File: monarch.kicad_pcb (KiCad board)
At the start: 2 copper layers, 159.6 x 123.3 mm, 137 parts, among them J1 USB_C_Receptacle_USB2.0, J2 USB_C_Receptacle_USB2.0, J3 OLED, SW1 SW_PUSH, SW10 SW_PUSH, SW11 SW_PUSH, SW12 SW_PUSH, SW13 SW_PUSH, SW14 SW_PUSH, SW15 SW_PUSH, SW16 SW_PUSH, SW17 SW_PUSH, SW18 SW_PUSH, SW19 Rotary_Encoder, SW2 SW_PUSH, SW20 SW_PUSH, SW21 SW_PUSH, SW22 SW_PUSH, SW23 SW_PUSH, SW24 SW_PUSH, SW3 SW_PUSH, SW4 SW_PUSH, SW5 SW_PUSH, SW6 SW_PUSH, SW7 SW_PUSH, SW8 SW_PUSH, SW9 SW_PUSH, U1 ATMEGA32U4, U2 MIC5219-5.0YMM, X1 16Mhz

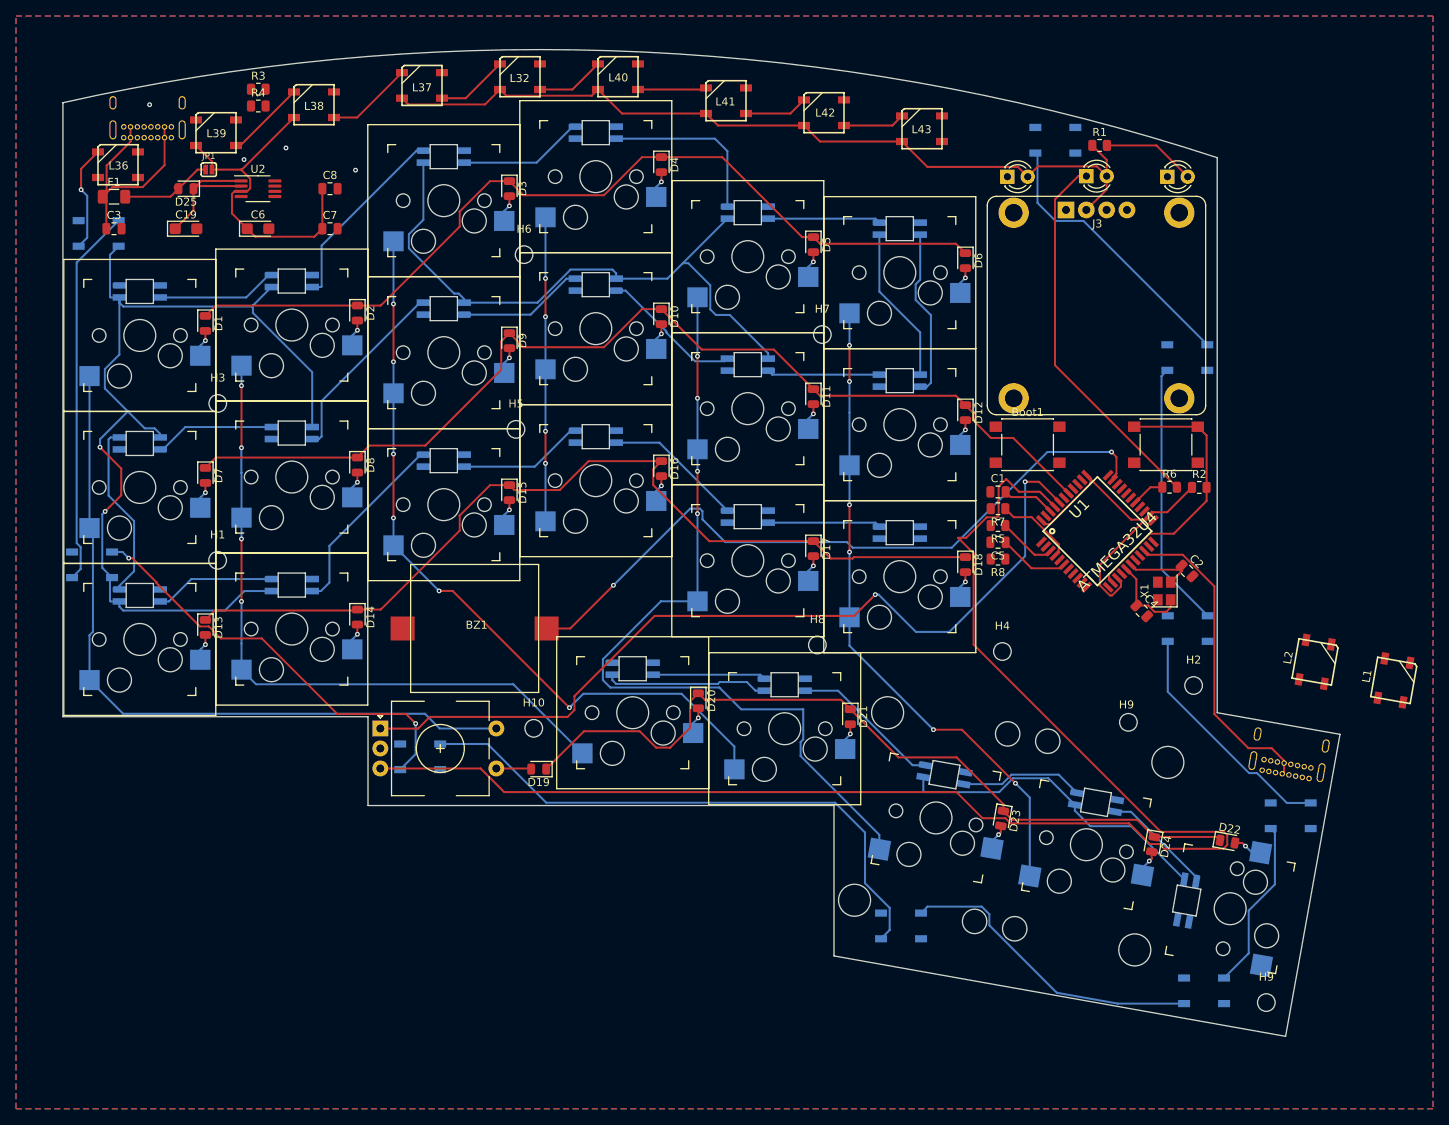
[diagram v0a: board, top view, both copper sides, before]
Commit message: plate edge case
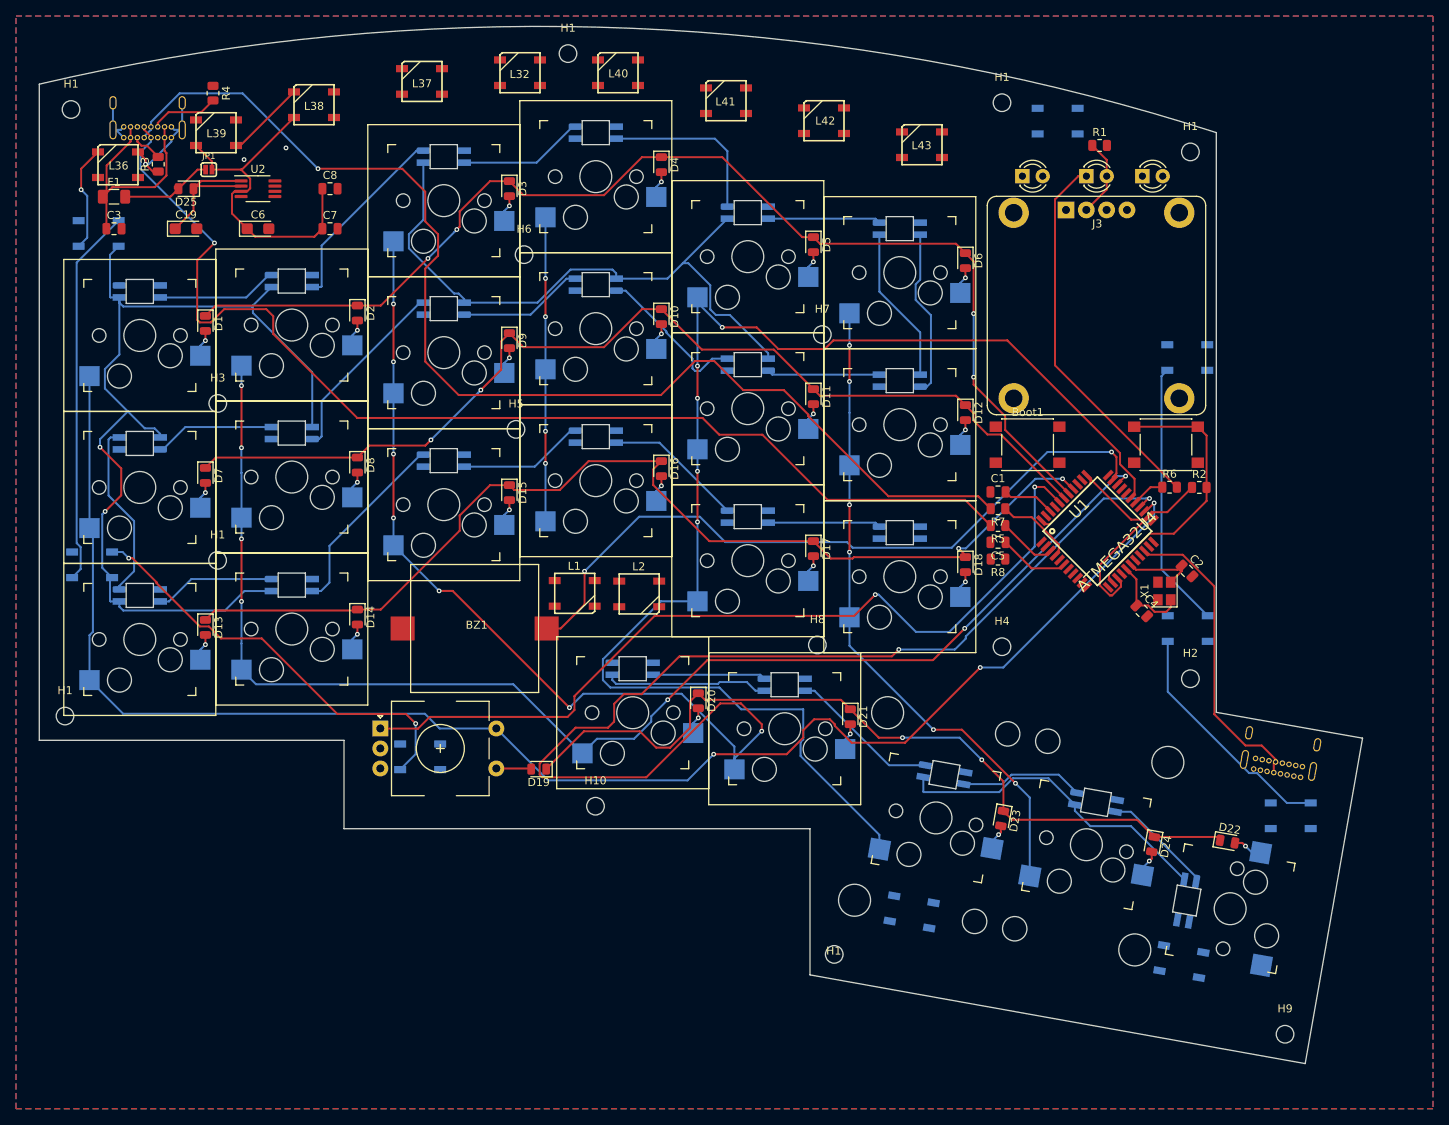
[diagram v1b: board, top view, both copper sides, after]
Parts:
- removed the H9 at (165.0, 126.7)
- removed the H9 at (147.8, 91.7)
- added H1: Hole, MountingHole:MountingHole_2.2mm_M2, F.Cu at (132.0, 14.2)
- added H1: Hole, MountingHole:MountingHole_2.2mm_M2, F.Cu at (155.6, 20.4)
- added H1: Hole, MountingHole:MountingHole_2.2mm_M2, F.Cu at (111.0, 120.7)
- added H1: Hole, MountingHole:MountingHole_2.2mm_M2, F.Cu at (14.9, 90.9)
- added H1: Hole, MountingHole:MountingHole_2.2mm_M2, F.Cu at (15.6, 15.1)
- added H1: Hole, MountingHole:MountingHole_2.2mm_M2, F.Cu at (77.8, 8.11)
- added H9: Hole, MountingHole:MountingHole_2.2mm_M2, F.Cu at (167.4, 130.7)
- moved L1 103.0 mm to (78.6, 75.6), turned to 0 degrees
- moved L2 84.9 mm to (86.7, 75.7), turned to 0 degrees
- moved R3 15.6 mm to (26.5, 21.9), turned to 90 degrees
- moved H10 12.4 mm to (81.2, 102.2)
- moved R4 5.89 mm to (33.4, 13.1), turned to 270 degrees
- moved L7 4.63 mm to (154.4, 121.6), turned to 350 degrees
- moved RED1 3.13 mm to (149.6, 23.4)
- moved L3 2.41 mm to (138.9, 16.6)
- moved L8 2.20 mm to (120.7, 115.4), turned to 350 degrees
- moved L43 2.00 mm to (122.0, 19.5)
- moved D26 1.88 mm to (134.6, 23.4)
- moved J2 1.07 mm to (163.5, 97.5)
- moved L42 1.00 mm to (109.8, 16.5)
- moved H2 0.94 mm to (155.6, 86.2)
- moved H4 0.60 mm to (132.0, 82.2)
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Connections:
- D1 pad 1: A3 -> A2
- D10 pad 1: A2 -> A3
- D11 pad 1: A2 -> A3
- D12 pad 1: A2 -> A3
- D2 pad 1: A3 -> A2
- D3 pad 1: A3 -> A2
- D4 pad 1: A3 -> A2
- D5 pad 1: A3 -> A2
- D6 pad 1: A3 -> A2
- D7 pad 1: A2 -> A3
- D8 pad 1: A2 -> A3
- D9 pad 1: A2 -> A3
- J2 pad A5: +5V -> GND
- J2 pad B5: +5V -> GND
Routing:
- net A5: track 185.9 -> 0.00 mm
- net Net-(J1-PadA6): track 0.00 -> 147.7 mm, vias 0 -> 1
- net Net-(J1-PadA7): track 0.00 -> 142.3 mm, vias 0 -> 1
- net COL2: track 95.3 -> 229.6 mm, vias 6 -> 9
- net COL0: track 91.7 -> 196.7 mm, vias 0 -> 3
- net VCC: track 468.2 -> 372.8 mm
- net COL1: track 85.0 -> 169.1 mm, vias 4 -> 7
- net Net-(L33-Pad3): track 72.7 -> 0.00 mm
- net COL4: track 103.7 -> 172.4 mm, vias 4 -> 5
- net Net-(L7-Pad1): track 38.6 -> 0.00 mm
- net Net-(L3-Pad1): track 34.9 -> 0.00 mm
- net GND: track 0.00 -> 22.1 mm
- net Net-(L6-Pad1): track 21.5 -> 0.00 mm
- net A1: track 113.2 -> 133.0 mm, vias 0 -> 2
- net A3: track 110.8 -> 129.4 mm, vias 0 -> 2
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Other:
- board size 159.6 x 123.3 mm -> 165.4 x 129.6 mm
